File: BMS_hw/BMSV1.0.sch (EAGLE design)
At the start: 201 parts, among them IC1 MC33771BEP, IC2 SFH6156, IC3 MIC28515V1, IC4 FOD8384-COC, IC5 FOD8384-COC, IC6 FOD8384-COC, J2 NTC, Q1 IRLML5203, Q2 IRLML5203, T1 IPT020N10N3V1, T2 IPT020N10N3V1, T3 IPT020N10N3V1, T4 IPT020N10N3V1, X1 87758-2016, X2 87758-1816, X4 87758-2016

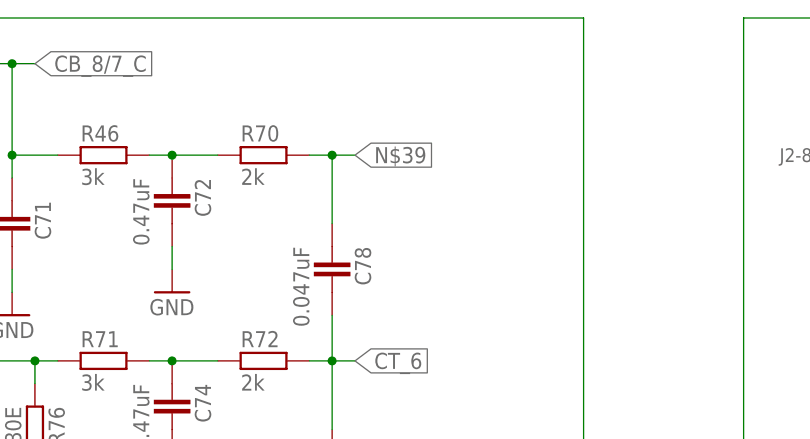
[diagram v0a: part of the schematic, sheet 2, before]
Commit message: board finnnnalo
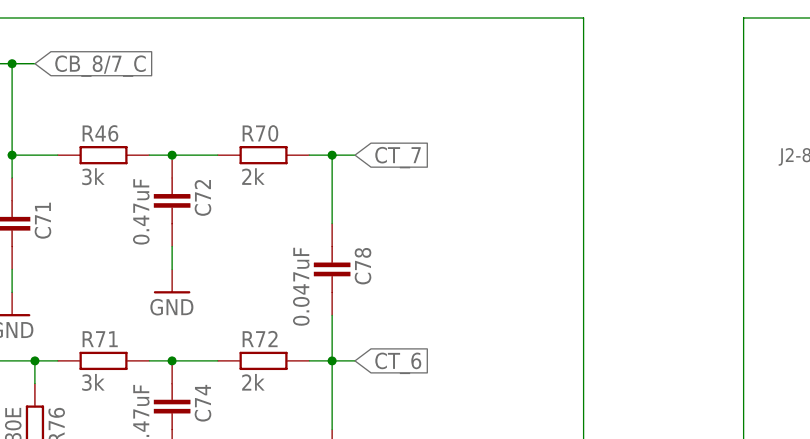
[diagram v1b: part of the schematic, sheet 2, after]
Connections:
- removed net N$39: C78.1, R70.2
- net CT_7: now also C78.1, R70.2
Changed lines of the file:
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@@
 </segment>
 </net>
-<net name="N$39" class="0">
+<net name="CT_7" class="0">
 <segment>
 <pinref part="R70" gate="G$1" pin="2"/>
